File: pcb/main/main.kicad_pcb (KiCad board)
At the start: 2 copper layers, 40.6 x 64.1 mm, 67 parts, among them J1 USB_C_Receptacle_USB2.0, J12 OLED, J13 trackball, J14 OLED, J2 RJ45, J3 RJ45, J4 STLink, J5 ROW, J6 COL, SW1 SW_SPDT, SW2 SW_SPDT, SW3 RESET, U1 STM32F401RETx, U2 NATLINEAR XT1861B332MR-G, U3 PCA9306DC1, U4 HT7727, Y1 Crystal_8MHz, Y2 Crystal_32.768MHz

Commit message: flat key
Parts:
- removed C1, C14, C15, C18, C19, C2, C21, C22, C23, C24, C25, C3, C4, C5: 0.1uF, Capacitor_SMD:C_0402_1005Metric
- removed C10, C11, C12, C9: C, Capacitor_SMD:C_0402_1005Metric
- removed C13, C16, C17, C20, C6: 1uF, Capacitor_SMD:C_0402_1005Metric
- removed C7: 10nF, Capacitor_SMD:C_0402_1005Metric
- removed C8: 4.7uF, Capacitor_SMD:C_0402_1005Metric
- removed F1: Polyfuse, Fuse:Fuse_0603_1608Metric
- removed J12, J14: OLED, folivora:OLED
- removed J13: trackball, Connector_JST:JST_PH_B5B-PH-K_1x05_P2.00mm_Vertical
- removed J3: RJ45, folivora:RJ45_rev
- removed J4: STLink, Connector_PinHeader_1.27mm:PinHeader_2x07_P1.27mm_Vertical
- removed J5: ROW, Connector_JST:JST_PH_B5B-PH-K_1x05_P2.00mm_Vertical
- removed J6: COL, Connector_JST:JST_PH_B6B-PH-K_1x06_P2.00mm_Vertical
- removed R1, R2, R39, R4, R5, R6, R7: R, Resistor_SMD:R_0402_1005Metric
- removed R24, R40: 10, Resistor_SMD:R_0402_1005Metric
- removed R41: 5.1k, Resistor_SMD:R_0402_1005Metric
- removed REF_M1 (x3), REF_M2, REF_M3, REF_M4, REF_M5, REF_M6: MountingHole_2.2mm_M2, MountingHole:MountingHole_2.2mm_M2
- removed U1: STM32F401RETx, Package_QFP:LQFP-64_10x10mm_P0.5mm
- removed U2: NATLINEAR XT1861B332MR-G, Package_TO_SOT_SMD:SOT-23
- removed U3: PCA9306DC1, Package_SO:VSSOP-8_2.3x2mm_P0.5mm
- removed U4: HT7727, Package_TO_SOT_SMD:SOT-23
- removed Y1: Crystal_8MHz, Crystal:Crystal_SMD_2520-4Pin_2.5x2.0mm
- removed Y2: Crystal_32.768MHz, Crystal:Crystal_SMD_2520-4Pin_2.5x2.0mm
- added D10: D, Diode_SMD:D_SOD-123, F.Cu at (134.6, 149.9)
- added D11: D, Diode_SMD:D_SOD-123, F.Cu at (152.4, 149.9)
- added D12: D, Diode_SMD:D_SOD-123, F.Cu at (171.4, 149.9)
- added D13: D, Diode_SMD:D_SOD-123, F.Cu at (85.1, 168.9)
- added D14: D, Diode_SMD:D_SOD-123, F.Cu at (101.6, 168.9)
- added D15: D, Diode_SMD:D_SOD-123, F.Cu at (120.7, 168.9)
- added D16: D, Diode_SMD:D_SOD-123, F.Cu at (139.7, 168.9)
- added D17: D, Diode_SMD:D_SOD-123, F.Cu at (158.8, 168.9)
- added D18: D, Diode_SMD:D_SOD-123, F.Cu at (177.8, 168.9)
- added D19: D, Diode_SMD:D_SOD-123, F.Cu at (68.6, 193.0)
- added D20: D, Diode_SMD:D_SOD-123, F.Cu at (87.6, 188.0)
- added D21: D, Diode_SMD:D_SOD-123, F.Cu at (106.7, 188.0)
- added D22: D, Diode_SMD:D_SOD-123, F.Cu at (124.5, 188.0)
- added D23: D, Diode_SMD:D_SOD-123, F.Cu at (143.5, 188.0)
- added D24: D, Diode_SMD:D_SOD-123, F.Cu at (163.8, 188.0)
- added D25: D, Diode_SMD:D_SOD-123, B.Cu at (72.4, 129.5)
- added D26: D, Diode_SMD:D_SOD-123, B.Cu at (91.4, 129.5)
- added D27: D, Diode_SMD:D_SOD-123, B.Cu at (109.2, 129.5)
- added D28: D, Diode_SMD:D_SOD-123, B.Cu at (129.5, 129.5)
- added D29: D, Diode_SMD:D_SOD-123, B.Cu at (148.6, 129.5)
- added D30: D, Diode_SMD:D_SOD-123, B.Cu at (167.6, 129.5)
- added D31: D, Diode_SMD:D_SOD-123, B.Cu at (78.7, 149.9)
- added D32: D, Diode_SMD:D_SOD-123, B.Cu at (96.5, 149.9)
- added D33: D, Diode_SMD:D_SOD-123, B.Cu at (115.6, 149.9)
- added D34: D, Diode_SMD:D_SOD-123, B.Cu at (134.6, 149.9)
- added D35: D, Diode_SMD:D_SOD-123, B.Cu at (152.4, 149.9)
- added D36: D, Diode_SMD:D_SOD-123, B.Cu at (171.4, 149.9)
- added D37: D, Diode_SMD:D_SOD-123, B.Cu at (85.1, 168.9)
- added D38: D, Diode_SMD:D_SOD-123, B.Cu at (101.6, 168.9)
- added D39: D, Diode_SMD:D_SOD-123, B.Cu at (120.7, 168.9)
- added D40: D, Diode_SMD:D_SOD-123, B.Cu at (139.7, 168.9)
- added D41: D, Diode_SMD:D_SOD-123, B.Cu at (158.8, 168.9)
- added D42: D, Diode_SMD:D_SOD-123, B.Cu at (177.8, 168.9)
- added D43: D, Diode_SMD:D_SOD-123, B.Cu at (68.6, 193.0)
- added D44: D, Diode_SMD:D_SOD-123, B.Cu at (87.6, 188.0)
- added D45: D, Diode_SMD:D_SOD-123, B.Cu at (106.7, 188.0)
- added D46: D, Diode_SMD:D_SOD-123, B.Cu at (124.5, 188.0)
- added D47: D, Diode_SMD:D_SOD-123, B.Cu at (143.5, 188.0)
- added D48: D, Diode_SMD:D_SOD-123, B.Cu at (163.8, 188.0)
- added D6: D, Diode_SMD:D_SOD-123, F.Cu at (167.6, 129.5)
- added D7: D, Diode_SMD:D_SOD-123, F.Cu at (78.7, 149.9)
- added D8: D, Diode_SMD:D_SOD-123, F.Cu at (96.5, 149.9)
- added D9: D, Diode_SMD:D_SOD-123, F.Cu at (115.6, 149.9)
- added REF**: MountingHole_2.2mm_M2, MountingHole:MountingHole_2.2mm_M2, F.Cu at (128.3, 168.3)
- added REF**: MountingHole_2.2mm_M2, MountingHole:MountingHole_2.2mm_M2, F.Cu at (67.3, 201.3)
- added REF**: MountingHole_2.2mm_M2, MountingHole:MountingHole_2.2mm_M2, F.Cu at (71.1, 145.4)
- added REF**: MountingHole_2.2mm_M2, MountingHole:MountingHole_2.2mm_M2, F.Cu at (188.6, 146.7)
- added REF**: MountingHole_2.2mm_M2, MountingHole:MountingHole_2.2mm_M2, F.Cu at (186.7, 194.3)
- added SW10: K42, folivora:Kailh_choc_V2, F.Cu at (143.5, 158.8)
- added SW11: K52, folivora:Kailh_choc_V2, F.Cu at (162.6, 158.8)
- added SW12: K62, folivora:Kailh_choc_V2, F.Cu at (181.6, 158.8)
- added SW13: K13, folivora:Kailh_choc_V2, F.Cu at (91.4, 177.8)
- added SW14: K23, folivora:Kailh_choc_V2, F.Cu at (110.5, 177.8)
- added SW15: K33, folivora:Kailh_choc_V2, F.Cu at (129.5, 177.8)
- added SW16: K43, folivora:Kailh_choc_V2, F.Cu at (148.6, 177.8)
- added SW17: K53, folivora:Kailh_choc_V2, F.Cu at (167.6, 177.8)
- added SW18: K63, folivora:Kailh_choc_V2, F.Cu at (186.7, 177.8)
- added SW19: K14, folivora:Kailh_choc_V2, F.Cu at (77.5, 196.8)
- added SW20: K24, folivora:Kailh_choc_V2, F.Cu at (96.5, 196.8)
- added SW21: K34, folivora:Kailh_choc_V2, F.Cu at (115.6, 196.8)
- added SW22: K44, folivora:Kailh_choc_V2, F.Cu at (134.6, 196.8)
- added SW23: K54, folivora:Kailh_choc_V2, F.Cu at (153.7, 196.8)
- added SW24: K64, folivora:Kailh_choc_V2, F.Cu at (172.7, 196.8)
- added SW4: K41, folivora:Kailh_choc_V2, F.Cu at (138.4, 139.7)
- added SW5: K51, folivora:Kailh_choc_V2, F.Cu at (157.5, 139.7)
- added SW6: K61, folivora:Kailh_choc_V2, F.Cu at (176.6, 139.7)
- added SW7: K12, folivora:Kailh_choc_V2, F.Cu at (86.4, 158.8)
- added SW8: K22, folivora:Kailh_choc_V2, F.Cu at (105.4, 158.8)
- added SW9: K32, folivora:Kailh_choc_V2, F.Cu at (124.5, 158.8)
- D1, D4: value SBD -> D
- D2: value Error -> D; footprint LED_SMD:LED_0603_1608Metric -> Diode_SMD:D_SOD-123
- D3: value Status -> D; footprint LED_SMD:LED_0603_1608Metric -> Diode_SMD:D_SOD-123
- D5: value LED_USB -> D; footprint LED_SMD:LED_0603_1608Metric -> Diode_SMD:D_SOD-123
- J1: value USB_C_Receptacle_USB2.0 -> Conn_01x10_MountingPin; footprint Connector_USB:USB_C_Receptacle_HRO_TYPE-C-31-M-12 -> Connector_FFC-FPC:TE_1-84952-0_1x10-1MP_P1.0mm_Horizontal
- J2: value RJ45 -> Conn_01x10_MountingPin; footprint folivora:RJ45_rev -> Connector_FFC-FPC:TE_1-84952-0_1x10-1MP_P1.0mm_Horizontal; moved to B.Cu
- SW1: value SW_SPDT -> K11; footprint Button_Switch_SMD:SW_SPDT_PCM12 -> folivora:Kailh_choc_V2
- SW2: value SW_SPDT -> K21; footprint Button_Switch_SMD:SW_SPDT_PCM12 -> folivora:Kailh_choc_V2
- SW3: value RESET -> K31; footprint Button_Switch_SMD:SW_SPST_EVQP7C -> folivora:Kailh_choc_V2
- moved J1 243.4 mm to (74.9, 177.8), turned to 270 degrees
- moved D5 231.9 mm to (148.6, 129.5), turned to 0 degrees
- moved SW3 226.5 mm to (119.4, 139.7), turned to 0 degrees
- moved D3 214.0 mm to (109.2, 129.5), turned to 0 degrees
- moved D2 206.0 mm to (91.4, 129.5), turned to 0 degrees
- moved SW1 200.9 mm to (81.3, 139.7), turned to 0 degrees
- moved SW2 200.7 mm to (100.3, 139.7), turned to 0 degrees
- moved J2 199.5 mm to (74.9, 177.8), turned to 90 degrees
- moved D4 194.5 mm to (129.5, 129.5), turned to 0 degrees
- moved D1 177.3 mm to (72.4, 129.5), turned to 0 degrees
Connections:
- D1 pad 1: Net-(C13-Pad1) -> /ROW1
- D1 pad 2: +3V3 -> Net-(D1-Pad2)
- D2 pad 1: /LED_ERROR -> /ROW1
- D3 pad 1: /LED_STATUS -> /ROW1
- D3 pad 2: Net-(D3-Pad2) -> Net-(D27-Pad2)
- D4 pad 1: Net-(C13-Pad1) -> /ROW1
- D4 pad 2: +2V8 -> Net-(D28-Pad2)
- D5 pad 1: GND -> /ROW1
- J2 pad 1: /MISO -> /ROW1
- J2 pad 2: /MISO -> /ROW2
- J2 pad 3: /MOSI -> /ROW3
- J2 pad 4: /SCLK -> /ROW4
- J2 pad 5: VBUS -> /COL1
- J2 pad 6: /MOSI -> /COL2
- J2 pad 7: /SS -> /COL3
- J2 pad 8: GND -> /COL4
- SW1 pad 1: Net-(C23-Pad1) -> /COL1
- SW1 pad 2: /BOOT0 -> Net-(D1-Pad2)
- SW2 pad 1: Net-(C22-Pad1) -> /COL2
- SW2 pad 2: /BOOT1 -> Net-(D2-Pad2)
- SW3 pad 1: GND -> /COL3
- SW3 pad 2: /NRST -> Net-(D27-Pad2)
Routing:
- net /COL6: track 15.1 -> 250.9 mm
- net GND: track 265.8 -> 38.4 mm, vias 14 -> 3
- net /COL5: track 15.7 -> 230.0 mm
- net /COL4: track 15.1 -> 202.8 mm
- net +3V3: track 178.3 -> 0.00 mm, vias 11 -> 0
- net /ROW1: track 6.86 -> 177.5 mm, vias 0 -> 9
- net /COL3: track 14.4 -> 179.6 mm
- net /COL2: track 14.2 -> 157.7 mm
- net /ROW2: track 7.21 -> 148.5 mm, vias 0 -> 9
- net /ROW4: track 9.60 -> 129.7 mm, vias 0 -> 8
- net /ROW3: track 7.95 -> 126.0 mm, vias 0 -> 9
- net /COL1: track 15.3 -> 132.0 mm
- net /NRST: track 85.9 -> 0.00 mm, vias 7 -> 0
- net VBUS: track 67.9 -> 0.00 mm, vias 3 -> 0
- net /SWCLK: track 47.8 -> 0.00 mm, vias 5 -> 0
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- removed copper zone on B.Cu, net GND
- removed copper zone on F.Cu, net GND
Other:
- board size 40.6 x 64.1 mm -> 130.8 x 78.7 mm

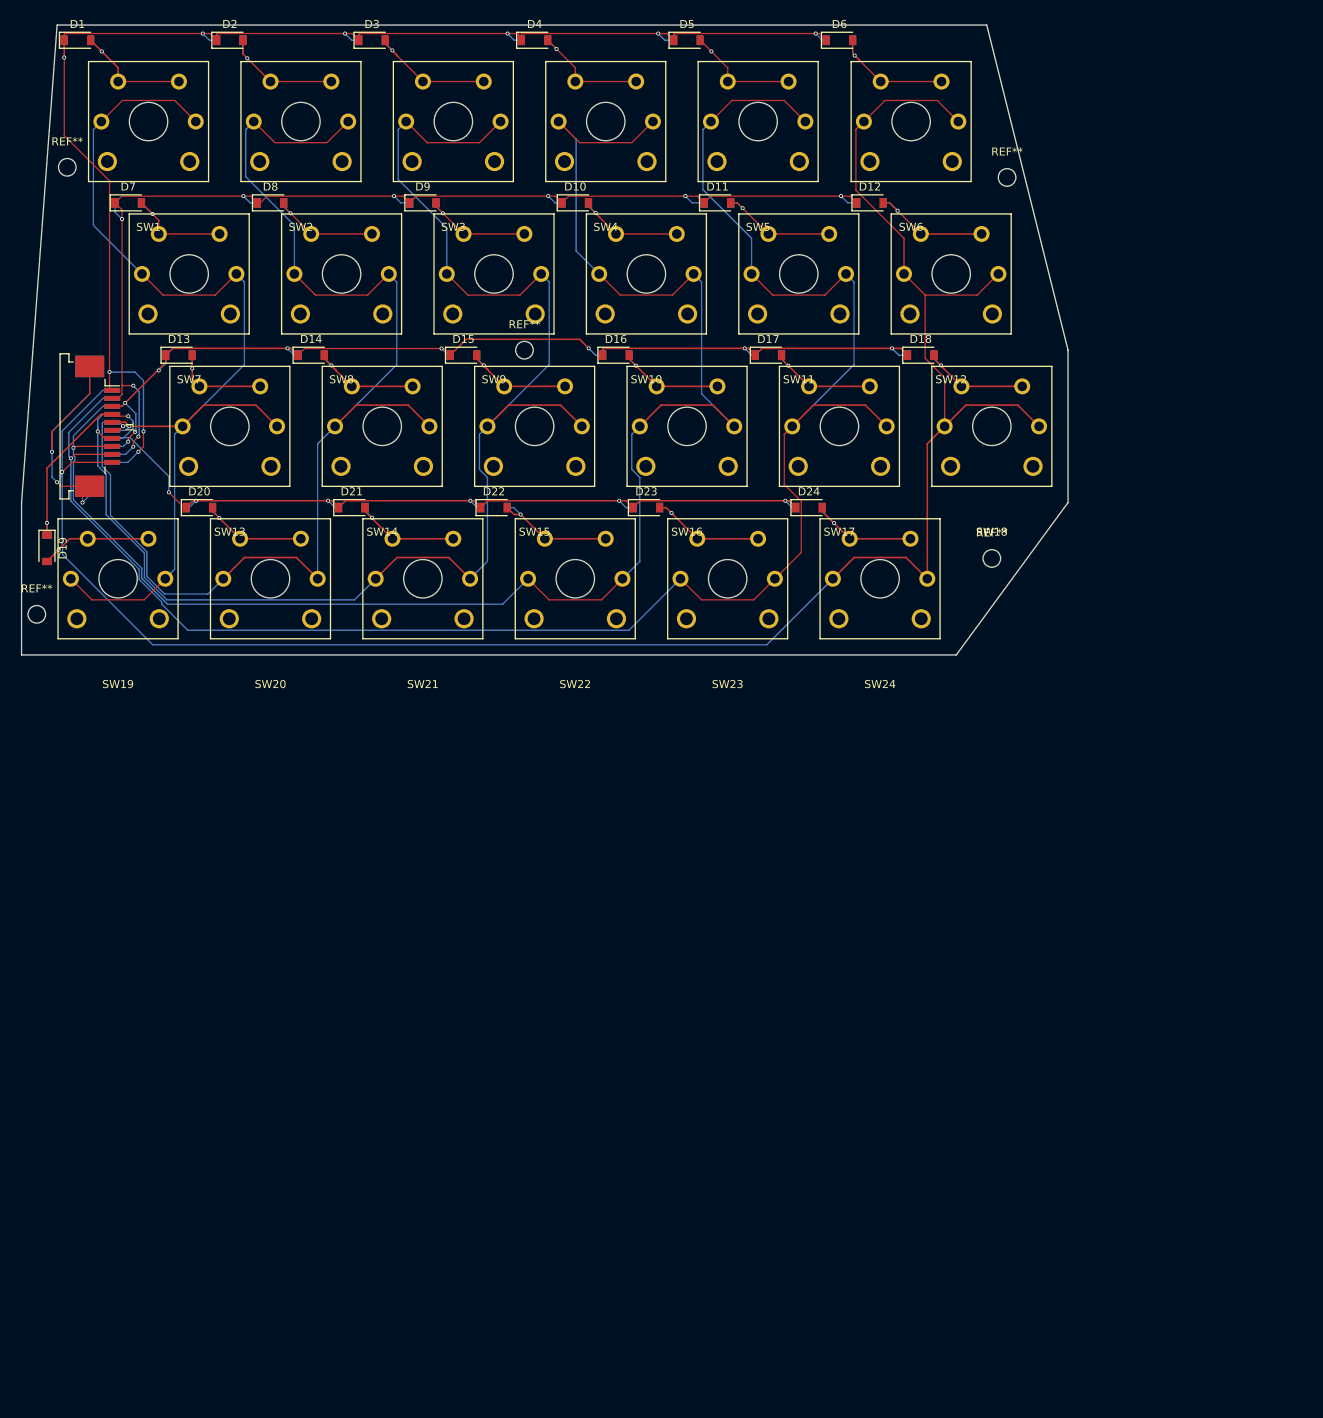
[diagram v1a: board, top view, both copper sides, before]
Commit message: right-hand
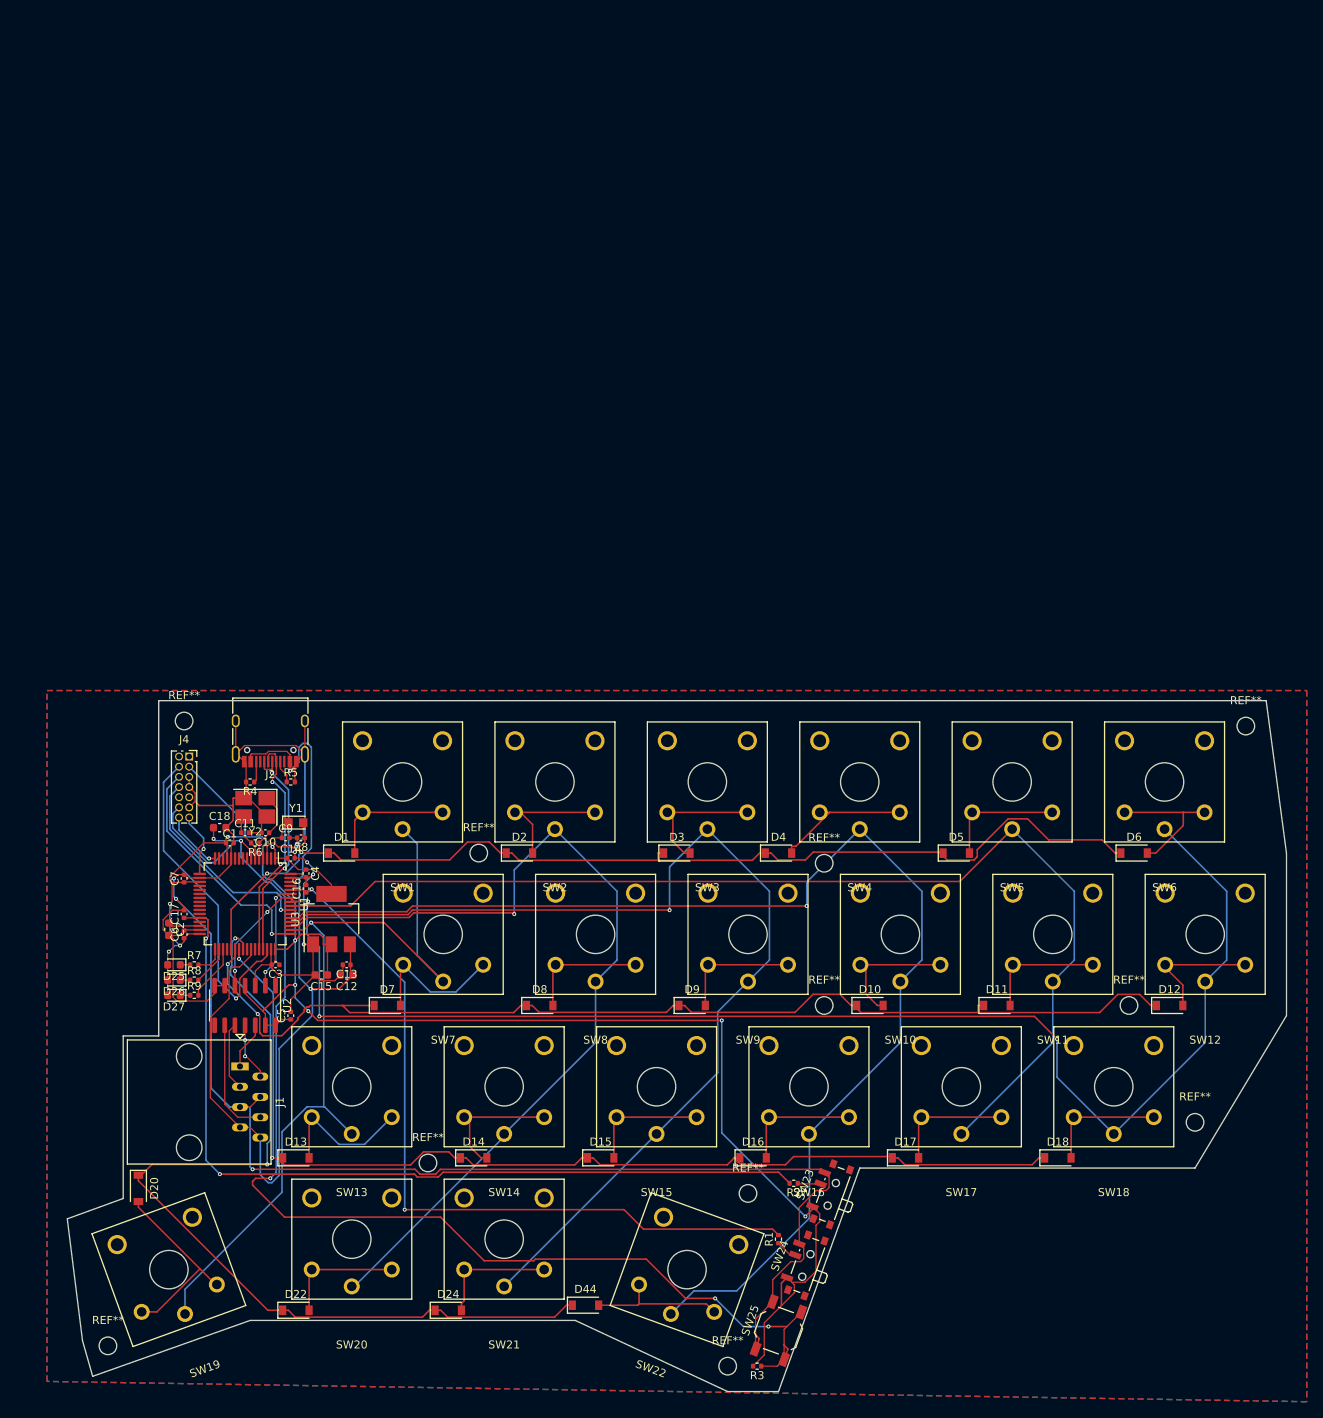
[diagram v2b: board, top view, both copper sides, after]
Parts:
- removed D19, D21, D23, D28, D29, D30, D31, D32, D33, D34, D35, D36, D37, D38, D39, D40, D41, D42, D43, D45, D46, D47, D48: D, Diode_SMD:D_SOD-123
- removed the REF** at (128.3, 168.3)
- removed the REF** at (67.3, 201.3)
- removed the REF** at (71.1, 145.4)
- removed the REF** at (188.6, 146.7)
- removed the REF** at (186.7, 194.3)
- added C1: 0.1uF, Capacitor_SMD:C_0402_1005Metric, F.Cu at (91.4, 229.9)
- added C10: 20pF, Capacitor_SMD:C_0402_1005Metric, F.Cu at (95.9, 228.6)
- added C11: 20pF, Capacitor_SMD:C_0402_1005Metric, F.Cu at (93.3, 228.6)
- added C12: 10uF, Capacitor_SMD:C_0603_1608Metric, F.Cu at (106.0, 246.4)
- added C13: 0.1uF, Capacitor_SMD:C_0402_1005Metric, F.Cu at (106.0, 245.1)
- added C14: 0.1uF, Capacitor_SMD:C_0402_1005Metric, F.Cu at (99.1, 231.8)
- added C15: 10uF, Capacitor_SMD:C_0603_1608Metric, F.Cu at (102.9, 246.4)
- added C16: 0.1uF, Capacitor_SMD:C_0402_1005Metric, F.Cu at (101.0, 235.6)
- added C17: 0.1uF, Capacitor_SMD:C_0402_1005Metric, F.Cu at (85.7, 238.8)
- added C18: 4.7uF, Capacitor_SMD:C_0603_1608Metric, F.Cu at (90.2, 228.0)
- added C2: 4.7uF, Capacitor_SMD:C_0603_1608Metric, F.Cu at (83.8, 240.7)
- added C3: 0.1uF, Capacitor_SMD:C_0402_1005Metric, F.Cu at (97.2, 245.1)
- added C4: 0.1uF, Capacitor_SMD:C_0402_1005Metric, F.Cu at (101.0, 233.7)
- added C5: 0.1uF, Capacitor_SMD:C_0402_1005Metric, F.Cu at (99.1, 251.5)
- added C6: 0.1uF, Capacitor_SMD:C_0402_1005Metric, F.Cu at (85.7, 241.3)
- added C7: 0.1uF, Capacitor_SMD:C_0402_1005Metric, F.Cu at (85.7, 234.3)
- added C8: 20pF, Capacitor_SMD:C_0402_1005Metric, F.Cu at (100.3, 229.2)
- added C9: 20pF, Capacitor_SMD:C_0402_1005Metric, F.Cu at (98.4, 229.2)
- added J4: Conn_02x07_Odd_Even, Connector_PinSocket_1.27mm:PinSocket_2x07_P1.27mm_Vertical, F.Cu at (86.4, 219.1)
- added R1: 220ohm, Resistor_SMD:R_0402_1005Metric, F.Cu at (160.0, 279.4)
- added R2: 220ohm, Resistor_SMD:R_0402_1005Metric, F.Cu at (161.9, 272.4)
- added R3: 10kohm, Resistor_SMD:R_0402_1005Metric, F.Cu at (157.4, 295.3)
- added R4: 5.1k, Resistor_SMD:R_0402_1005Metric, F.Cu at (94.0, 222.2)
- added R5: 5.1k, Resistor_SMD:R_0402_1005Metric, F.Cu at (99.1, 222.2)
- added R6: 1Mohm, Resistor_SMD:R_0402_1005Metric, F.Cu at (94.6, 229.9)
- added R7: 220ohm, Resistor_SMD:R_0402_1005Metric, F.Cu at (87.0, 245.1)
- added R8: 220ohm, Resistor_SMD:R_0402_1005Metric, F.Cu at (87.0, 247.0)
- added R9: 220ohm, Resistor_SMD:R_0402_1005Metric, F.Cu at (87.0, 248.9)
- added REF**: MountingHole_2.2mm_M2, MountingHole:MountingHole_2.2mm_M2, F.Cu at (85.7, 214.6)
- added REF**: MountingHole_2.2mm_M2, MountingHole:MountingHole_2.2mm_M2, F.Cu at (116.2, 269.9)
- added REF**: MountingHole_2.2mm_M2, MountingHole:MountingHole_2.2mm_M2, F.Cu at (76.2, 292.7)
- added REF**: MountingHole_2.2mm_M2, MountingHole:MountingHole_2.2mm_M2, F.Cu at (165.7, 250.2)
- added REF**: MountingHole_2.2mm_M2, MountingHole:MountingHole_2.2mm_M2, F.Cu at (156.2, 273.7)
- added REF**: MountingHole_2.2mm_M2, MountingHole:MountingHole_2.2mm_M2, F.Cu at (122.6, 231.1)
- added REF**: MountingHole_2.2mm_M2, MountingHole:MountingHole_2.2mm_M2, F.Cu at (165.7, 232.4)
- added REF**: MountingHole_2.2mm_M2, MountingHole:MountingHole_2.2mm_M2, F.Cu at (212.1, 264.8)
- added REF**: MountingHole_2.2mm_M2, MountingHole:MountingHole_2.2mm_M2, F.Cu at (218.4, 215.3)
- added REF**: MountingHole_2.2mm_M2, MountingHole:MountingHole_2.2mm_M2, F.Cu at (203.8, 250.2)
- added REF**: MountingHole_2.2mm_M2, MountingHole:MountingHole_2.2mm_M2, F.Cu at (153.7, 295.3)
- added SW25: RST, Button_Switch_SMD:SW_SPST_TL3342, F.Cu at (160.0, 290.8)
- added U1: STM32F401RETx, Package_QFP:LQFP-64_10x10mm_P0.5mm, F.Cu at (93.3, 237.5)
- added U2: ADM1491EBR, Package_SO:SOIC-14_3.9x8.7mm_P1.27mm, F.Cu at (93.3, 250.2)
- added U3: LD1117S33TR_SOT223, Package_TO_SOT_SMD:SOT-223-3_TabPin2, F.Cu at (104.1, 239.4)
- added Y1: 32.768kHz, Crystal:Crystal_SMD_2012-2Pin_2.0x1.2mm_HandSoldering, F.Cu at (99.7, 227.3)
- added Y2: 8MHz, Crystal:Crystal_SMD_3225-4Pin_3.2x2.5mm_HandSoldering, F.Cu at (94.6, 225.4)
- D25: value D -> STATUS0; footprint Diode_SMD:D_SOD-123 -> LED_SMD:LED_0603_1608Metric; moved to F.Cu
- D26: value D -> STATUS1; footprint Diode_SMD:D_SOD-123 -> LED_SMD:LED_0603_1608Metric; moved to F.Cu
- D27: value D -> STATUS2; footprint Diode_SMD:D_SOD-123 -> LED_SMD:LED_0603_1608Metric; moved to F.Cu
- D44: moved to F.Cu
- J1: value Conn_01x10_MountingPin -> RJ45; footprint Connector_FFC-FPC:TE_1-84952-0_1x10-1MP_P1.0mm_Horizontal -> folivora:RJ45_rev
- J2: value Conn_01x10_MountingPin -> USB_C_Receptacle_USB2.0; footprint Connector_FFC-FPC:TE_1-84952-0_1x10-1MP_P1.0mm_Horizontal -> Connector_USB:USB_C_Receptacle_HRO_TYPE-C-31-M-12; moved to F.Cu
- SW23: value K54 -> BOOT1; footprint folivora:Kailh_choc_V2 -> Button_Switch_SMD:SW_SPDT_PCM12
- SW24: value K64 -> BOOT0; footprint folivora:Kailh_choc_V2 -> Button_Switch_SMD:SW_SPDT_PCM12
- moved D27 121.9 mm to (84.5, 248.9), turned to 180 degrees
- moved D26 117.7 mm to (84.5, 247.0), turned to 180 degrees
- moved D25 116.2 mm to (84.5, 245.1), turned to 180 degrees
- moved D44 110.8 mm to (135.9, 287.7)
- moved D24 110.0 mm to (118.7, 288.3)
- moved D3 108.5 mm to (147.3, 231.1)
- moved D6 108.1 mm to (204.5, 231.1)
- moved D2 107.9 mm to (127.6, 231.1)
- moved D12 107.1 mm to (208.9, 250.2)
- moved D5 107.0 mm to (182.2, 231.1)
- moved D10 106.9 mm to (171.4, 250.2)
- moved D1 106.8 mm to (105.4, 231.1)
- moved D11 106.2 mm to (187.3, 250.2)
- moved D4 106.1 mm to (160.0, 231.1)
- moved D8 105.8 mm to (130.2, 250.2)
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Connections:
- D25 pad 1: /ROW1 -> Net-(D25-Pad1)
- D25 pad 2: Net-(D1-Pad2) -> +3V3
- D26 pad 1: /ROW1 -> Net-(D26-Pad1)
- D26 pad 2: Net-(D2-Pad2) -> +3V3
- D27 pad 1: /ROW1 -> Net-(D27-Pad1)
- D27 pad 2: Net-(D27-Pad2) -> +3V3
- D3 pad 2: Net-(D27-Pad2) -> Net-(D3-Pad2)
- D44 pad 2: Net-(D20-Pad2) -> Net-(D44-Pad2)
- J1 pad 1: /ROW1 -> /RX+
- J1 pad 2: /ROW2 -> /RX-
- J1 pad 3: /ROW3 -> /TX+
- J1 pad 4: /ROW4 -> GND
- J1 pad 5: /COL1 -> GND
- J1 pad 6: /COL2 -> /TX-
- J1 pad 7: /COL3 -> +5V
- J1 pad 8: /COL4 -> +5V
- SW19 pad 2: Net-(D19-Pad2) -> Net-(D20-Pad2)
- SW20 pad 2: Net-(D20-Pad2) -> Net-(D22-Pad2)
- SW21 pad 2: Net-(D21-Pad2) -> Net-(D24-Pad2)
- SW22 pad 2: Net-(D22-Pad2) -> Net-(D44-Pad2)
- SW23 pad 1: /COL5 -> +3V3
- SW24 pad 1: /COL6 -> +3V3
- SW24 pad 2: Net-(D24-Pad2) -> Net-(R1-Pad1)
- SW3 pad 2: Net-(D27-Pad2) -> Net-(D3-Pad2)
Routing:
- net GND: track 38.4 -> 300.1 mm, vias 3 -> 8
- net +3V3: track 0.00 -> 231.9 mm, vias 0 -> 10
- net /RST: track 0.00 -> 156.3 mm, vias 0 -> 5
- net +5V: track 0.00 -> 117.3 mm, vias 0 -> 2
- net /BOOT1: track 0.00 -> 107.9 mm, vias 0 -> 2
- net /BOOT0: track 0.00 -> 96.0 mm, vias 0 -> 2
- net /COL5: track 230.0 -> 141.3 mm, vias 1 -> 0
- net /COL6: track 250.9 -> 172.7 mm, vias 1 -> 3
- net /ROW1: track 177.5 -> 129.8 mm, vias 9 -> 2
- net /COL3: track 179.6 -> 134.2 mm
- net /COL4: track 202.8 -> 157.5 mm
- net /COL2: track 157.7 -> 115.7 mm
- net /SWDIO: track 0.00 -> 41.6 mm, vias 0 -> 1
- net /SWCLK: track 0.00 -> 29.9 mm, vias 0 -> 1
- net /D-: track 0.00 -> 28.7 mm, vias 0 -> 2
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- added copper zone on B.Cu, net GND
- added copper zone on F.Cu, net GND
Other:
- board size 130.8 x 78.7 mm -> 152.4 x 86.4 mm
